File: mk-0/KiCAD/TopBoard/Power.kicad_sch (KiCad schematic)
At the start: 33 parts, among them J3 USB_C_Receptacle_USB2.0_16P, J5 Raspberry_Pi_2_3, U10 SRV05-4, U11 AMS1117-1.2, U6 CAT24C256, U9 AMS1117-3.3

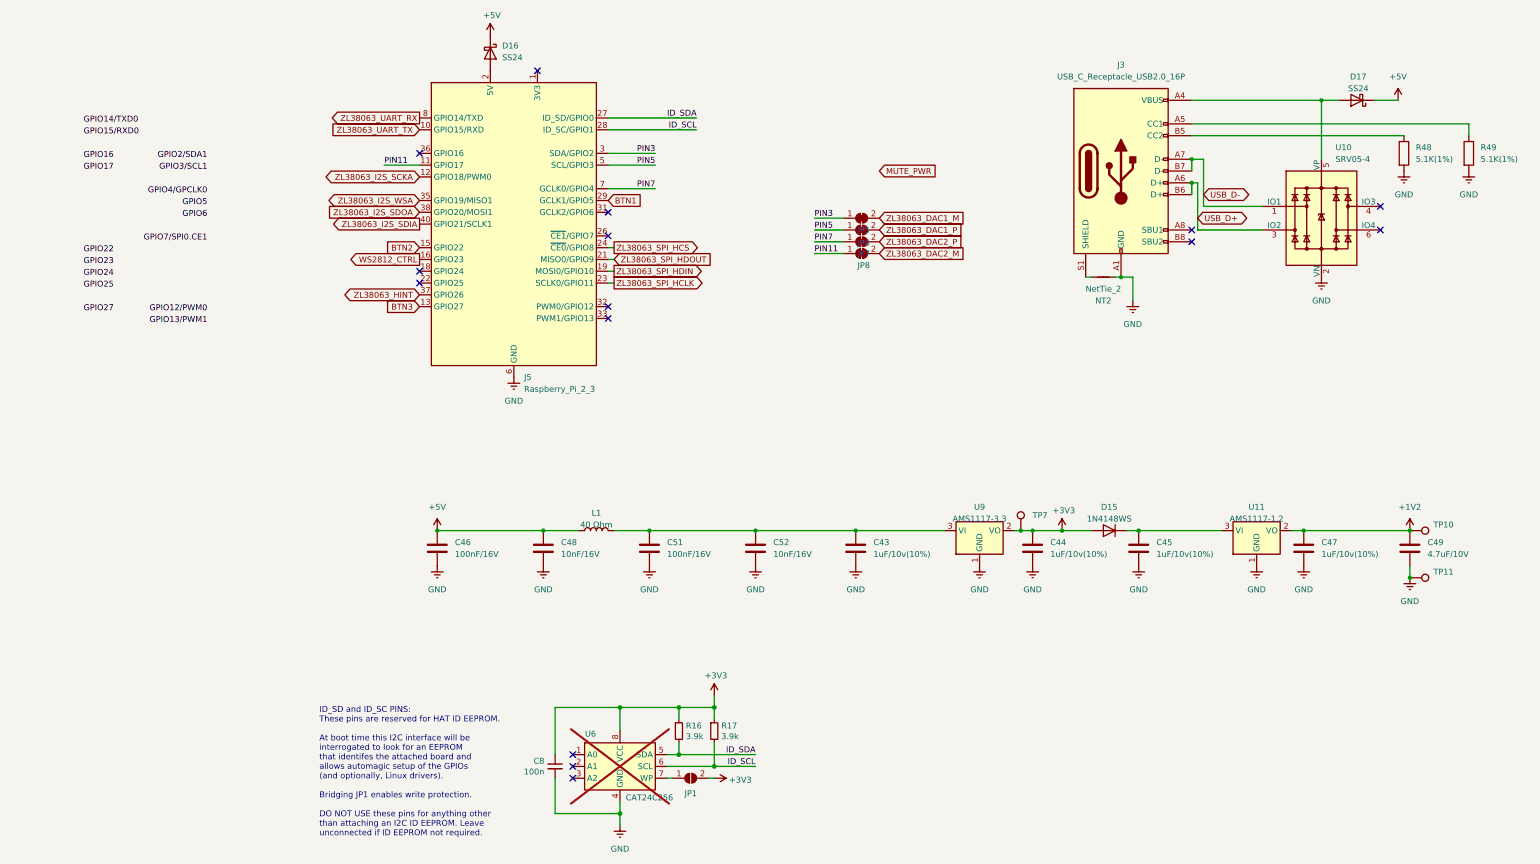
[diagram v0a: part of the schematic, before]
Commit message: Cleanup and naming of Touchpoints
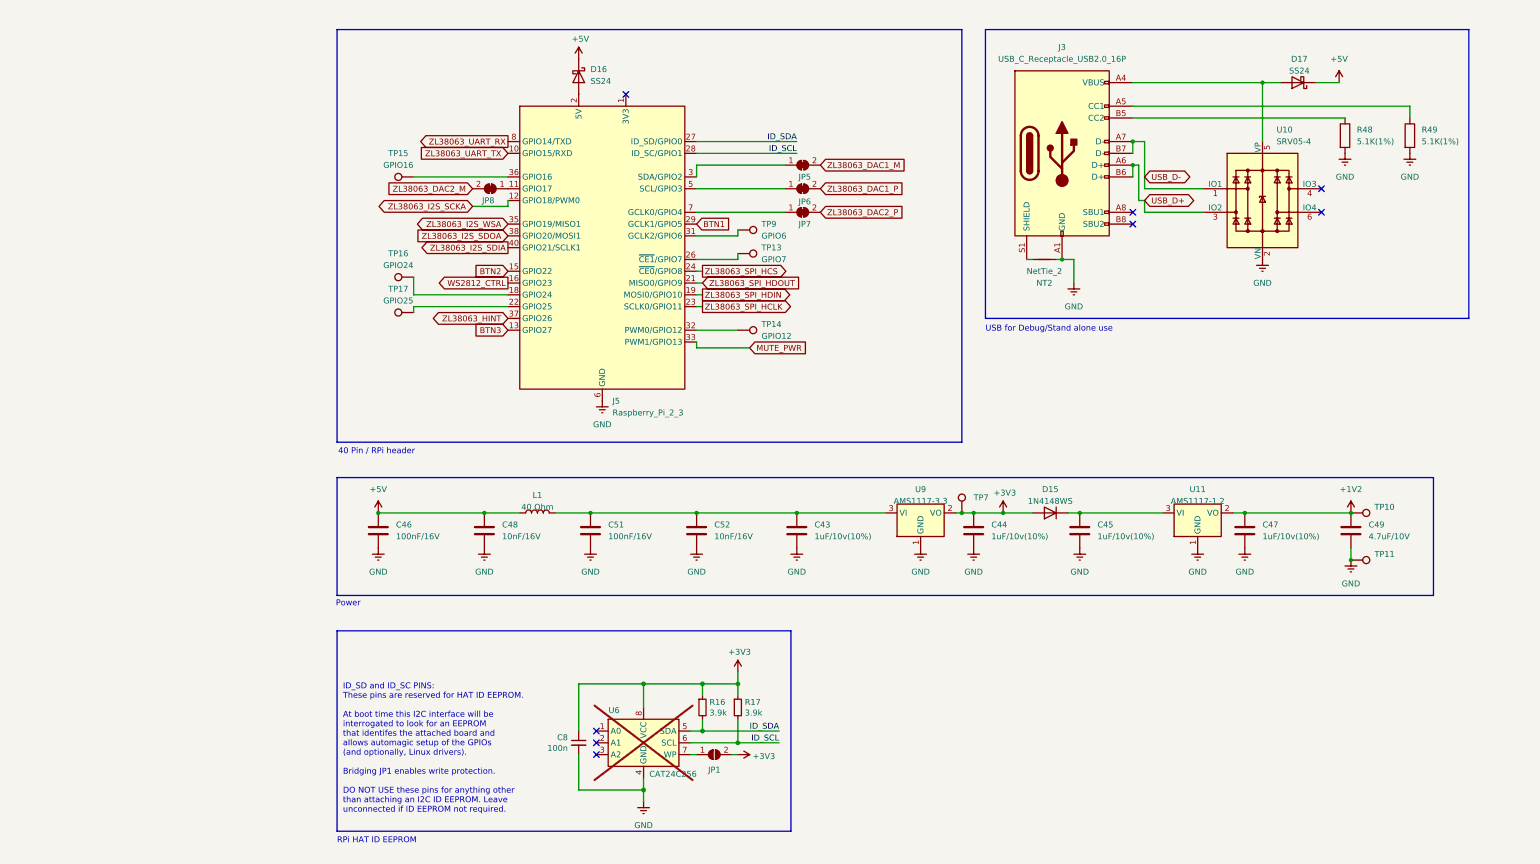
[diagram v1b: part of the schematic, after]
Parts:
- added TP13: GPIO7, TestPoint:TestPoint_Pad_D1.0mm, symbol Connector:TestPoint
- added TP14: GPIO12, TestPoint:TestPoint_Pad_D1.0mm, symbol Connector:TestPoint
- added TP15: GPIO16, TestPoint:TestPoint_Pad_D1.0mm, symbol Connector:TestPoint
- added TP16: GPIO24, TestPoint:TestPoint_Pad_D1.0mm, symbol Connector:TestPoint
- added TP17: GPIO25, TestPoint:TestPoint_Pad_D1.0mm, symbol Connector:TestPoint
- added TP9: GPIO6, TestPoint:TestPoint_Pad_D1.0mm, symbol Connector:TestPoint
- TP10: value TestPoint -> 1V2
- TP11: value TestPoint -> GND
- TP7: value TestPoint -> 3V3
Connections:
- net MUTE_PWR: now also J5.33 (PWM1/GPIO13)
- net at J5.18 (GPIO24): now also TP16.1
- net at J5.22 (GPIO25): now also TP17.1
- net at J5.26 (~{CE1}/GPIO7): now also TP13.1
- net at J5.31 (GCLK2/GPIO6): now also TP9.1
- net at J5.32 (PWM0/GPIO12): now also TP14.1
- net at J5.36 (GPIO16): now also TP15.1
- net PIN11: no longer names the net of J5.11 (GPIO17), JP8.1 (A)
- net PIN3: no longer names the net of J5.3 (SDA/GPIO2), JP5.1 (A)
- net PIN5: no longer names the net of J5.5 (SCL/GPIO3), JP6.1 (A)
- net PIN7: no longer names the net of J5.7 (GCLK0/GPIO4), JP7.1 (A)
- no-connect marks 15 -> 8
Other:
- note added: "40 Pin / RPi header"
- note added: "Power"
- note added: "RPi HAT ID EEPROM"
- note added: "USB for Debug/Stand alone use"
- moved on the sheet: C43, C44, C45, C46, C47, C48, C49, C51, C52, C8, D15, D16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
